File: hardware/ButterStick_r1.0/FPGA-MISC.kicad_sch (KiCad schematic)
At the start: 11 parts, among them U4 ECP5UM5G_85_CABGA381, X1 ASDMB

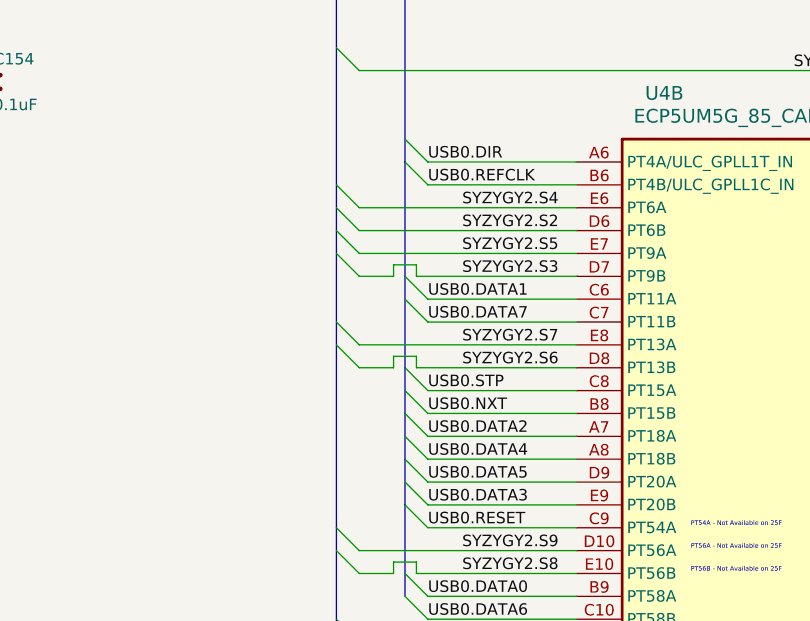
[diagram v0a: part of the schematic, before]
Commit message: hw.r1d0: Review complete, gerbers generated
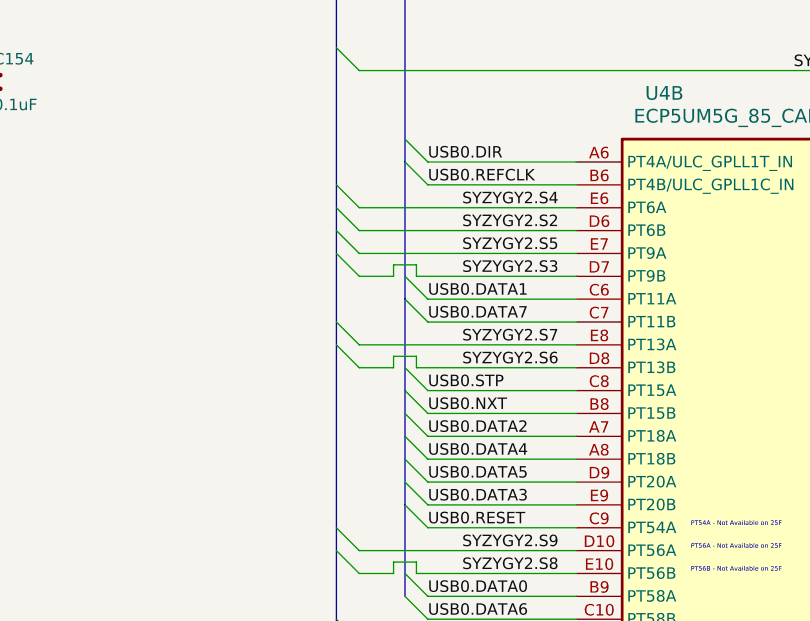
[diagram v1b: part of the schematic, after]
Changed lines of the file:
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@@
 (kicad_sch (version 20200618) (host eeschema "5.99.0-unknown-73168a9~101~ubuntu18.04.1")
-  (page 1 18)
+  (page 6 18)
   (paper "A4")
   (title_block
     (title "ButterStick")
-    (date "2020-07-16")
+    (date "2020-07-17")
     (rev "r1.0")
     (company "GsD")
@@
     (stroke (width 0) (type solid) (color 0 0 0 0))
   )
-  (bus (pts (xy 195.58 82.55) (xy 195.58 95.25))
-    (stroke (width 0) (type solid) (color 0 0 0 0))
-  )
-  (bus (pts (xy 195.58 95.25) (xy 195.58 105.41))
-    (stroke (width 0) (type solid) (color 0 0 0 0))
-  )
-  (bus (pts (xy 195.58 105.41) (xy 195.58 110.49))
-    (stroke (width 0) (type solid) (color 0 0 0 0))
-  )
-  (bus (pts (xy 195.58 110.49) (xy 195.58 115.57))
-    (stroke (width 0) (type solid) (color 0 0 0 0))
-  )
+  (bus (pts (xy 195.58 82.55) (xy 195.58 97.79))
+    (stroke (width 0) (type solid) (color 0 0 0 0))
+  )
+  (bus (pts (xy 195.58 97.79) (xy 195.58 107.95))
+    (stroke (width 0) (type solid) (color 0 0 0 0))
+  )
+  (bus (pts (xy 195.58 107.95) (xy 195.58 113.03))
+    (stroke (width 0) (type solid) (color 0 0 0 0))
+  )
+  (bus (pts (xy 195.58 113.03) (xy 195.58 115.57))
+    (stroke (width 0) (type solid) (color 0 0 0 0))
+  )
